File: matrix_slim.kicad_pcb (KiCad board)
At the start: 2 copper layers, 84 x 62.3 mm, 66 parts, among them J2 C168688, SW1 PG1316M, SW10 PG1316S, SW11 PG1316S, SW12 PG1316S, SW13 PG1316S, SW14 PG1316S, SW15 PG1316M, SW16 PG1316M, SW17 PG1316S, SW18 PG1316M, SW2 PG1316M, SW3 PG1316M, SW4 PG1316M, SW5 PG1316M, SW6 PG1316S, SW7 PG1316S, SW8 PG1316S, SW9 PG1316S, U1 nRF52840, U2 BQ24075RGT, U3 XC6220B331MR, Y1 FC-12M, Y2 23MHz XRCGB32M000F1H50R0

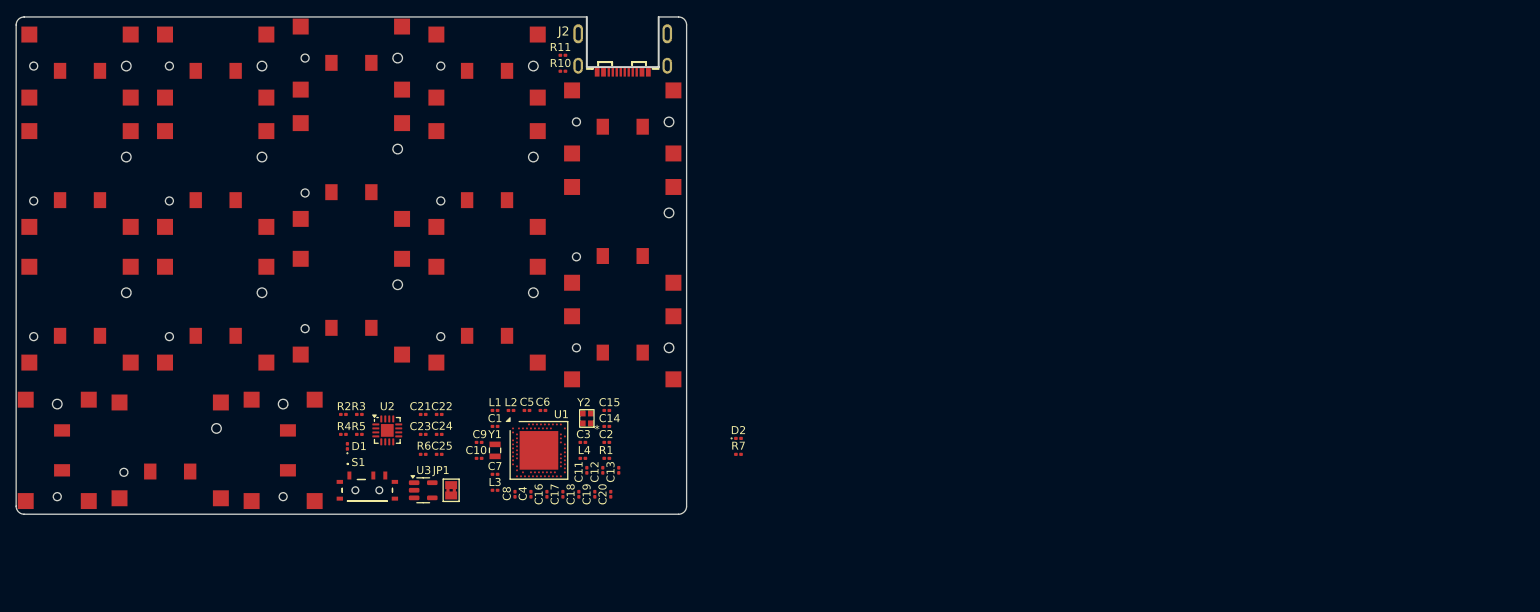
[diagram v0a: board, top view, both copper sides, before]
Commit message: Added base setup
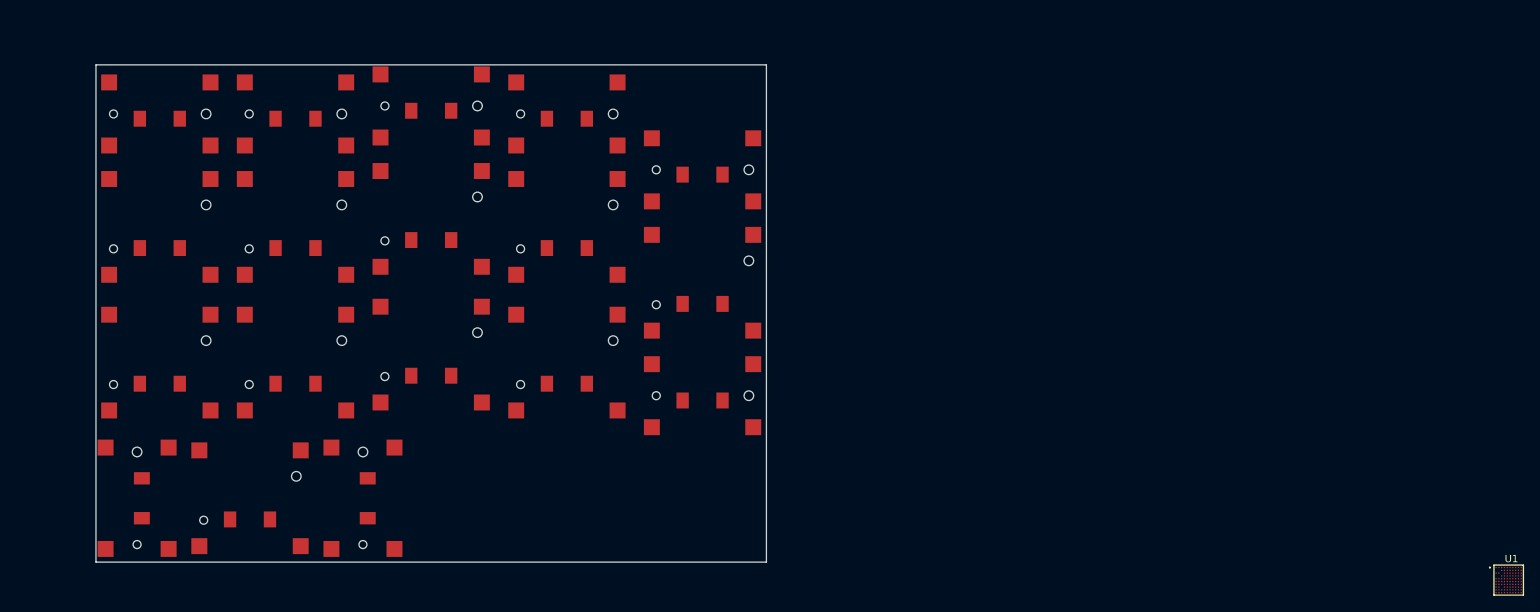
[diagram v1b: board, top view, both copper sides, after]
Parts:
- removed C1, C17, C18, C19: 100nF, Capacitor_SMD:C_0201_0603Metric
- removed C10, C14, C15, C9: 12pF, Capacitor_SMD:C_0201_0603Metric
- removed C11, C12: 1pF, Capacitor_SMD:C_0201_0603Metric
- removed C13: 1.5pF, Capacitor_SMD:C_0201_0603Metric
- removed C16, C21, C6: 1uF, Capacitor_SMD:C_0201_0603Metric
- removed C2: 100pF, Capacitor_SMD:C_0201_0603Metric
- removed C20, C22, C23, C4, C7, C8: 4.7uF, Capacitor_SMD:C_0201_0603Metric
- removed C24: 10uF, Capacitor_SMD:C_0201_0603Metric
- removed C25: 4.7nF, Capacitor_SMD:C_0201_0603Metric
- removed C3: 820pF, Capacitor_SMD:C_0201_0603Metric
- removed C5: 47nF, Capacitor_SMD:C_0201_0603Metric
- removed D1: RED, LED_SMD:LED_0201_0603Metric
- removed D2: BLUE, LED_SMD:LED_0201_0603Metric
- removed J2: C168688, custom_footprints:C168688
- removed JP1: Charge Boost, Jumper:SolderJumper-2_P1.3mm_Bridged2Bar_Pad1.0x1.5mm
- removed L1, L3: 10uH, Inductor_SMD:L_0201_0603Metric
- removed L2: 15nH, Inductor_SMD:L_0201_0603Metric
- removed L4: 3.9nH, Inductor_SMD:L_0201_0603Metric
- removed R1: 0, Resistor_SMD:R_0201_0603Metric
- removed R10, R11: 5.1k, Resistor_SMD:R_0201_0603Metric
- removed R2, R4, R5: 10k, Resistor_SMD:R_0201_0603Metric
- removed R3: 2k, Resistor_SMD:R_0201_0603Metric
- removed R6: 10M, Resistor_SMD:R_0201_0603Metric
- removed R7: 1k, Resistor_SMD:R_0201_0603Metric
- removed S1: MSK12C02, custom_footprints:MSK12C02
- removed U2: BQ24075RGT, Package_DFN_QFN:VQFN-16-1EP_3x3mm_P0.5mm_EP1.6x1.6mm
- removed U3: XC6220B331MR, Package_TO_SOT_SMD:SOT-23-5
- removed Y1: FC-12M, Crystal:Crystal_SMD_3215-2Pin_3.2x1.5mm
- removed Y2: 23MHz XRCGB32M000F1H50R0, custom_footprints:XRCGB32M000F1H01R0
- SW1, SW15, SW16, SW18, SW3, SW4, SW5: footprint custom_footprints:CPG1316M01D02 -> PG1316M:PG1316M
- SW10, SW11, SW12, SW13, SW14, SW17, SW7, SW8, SW9: footprint custom_footprints:CPG1316S01D02 -> PG1316S:PG1316S
- SW2: value PG1316M -> PG1316S; footprint custom_footprints:CPG1316M01D02 -> PG1316S:PG1316S
- SW6: value PG1316S -> PG1316M; footprint custom_footprints:CPG1316S01D02 -> PG1316M:PG1316M
- U1: value nRF52840 -> NRF52840-CKAA-R; footprint Package_DFN_QFN:Nordic_AQFN-73-1EP_7x7mm_P0.5mm -> NRF52840-CKAA-R:NRF52840-CKAA-R
- moved U1 122.6 mm to (207.0, 95.3)
- moved SW6 78.0 mm to (106.0, 43.9)
- moved SW2 21.3 mm to (38.0, 51.0)
- moved SW1 11.7 mm to (38.0, 36.9)
- moved SW10 11.7 mm to (106.0, 58.0)
- moved SW11 11.7 mm to (38.0, 68.0)
- moved SW12 11.7 mm to (55.0, 68.0)
- moved SW13 11.7 mm to (72.0, 67.0)
- moved SW14 11.7 mm to (89.0, 68.0)
- moved SW15 11.7 mm to (106.0, 72.2)
- moved SW16 11.7 mm to (35.1, 85.0)
- moved SW17 11.7 mm to (49.3, 85.0)
- moved SW18 11.7 mm to (63.5, 85.0)
- moved SW7 11.7 mm to (55.0, 51.0)
- moved SW8 11.7 mm to (72.0, 50.0)
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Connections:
- SW1 pad 2: SGND -> GND
- SW1 pad 3: FGND -> SGND
- SW10 pad 2: SGND -> GND
- SW10 pad 3: FGND -> SGND
- SW11 pad 2: SGND -> GND
- SW11 pad 3: FGND -> SGND
- SW12 pad 2: SGND -> GND
- SW12 pad 3: FGND -> SGND
- SW13 pad 2: SGND -> GND
- SW13 pad 3: FGND -> SGND
- SW14 pad 2: SGND -> GND
- SW14 pad 3: FGND -> SGND
- SW15 pad 2: SGND -> GND
- SW15 pad 3: FGND -> SGND
- SW16 pad 2: SGND -> GND
- SW16 pad 3: FGND -> SGND
- SW17 pad 2: SGND -> GND
- SW17 pad 3: FGND -> SGND
- SW18 pad 2: SGND -> GND
- SW18 pad 3: FGND -> SGND
- SW2 pad 2: SGND -> GND
- SW2 pad 3: FGND -> SGND
- SW3 pad 2: SGND -> GND
- SW3 pad 3: FGND -> SGND
- SW4 pad 2: SGND -> GND
- SW4 pad 3: FGND -> SGND
- SW5 pad 2: SGND -> GND
- SW5 pad 3: FGND -> SGND
- SW6 pad 2: SGND -> GND
- SW6 pad 3: FGND -> SGND
- SW7 pad 2: SGND -> GND
- SW7 pad 3: FGND -> SGND
- SW8 pad 2: SGND -> GND
- SW8 pad 3: FGND -> SGND
- SW9 pad 2: SGND -> GND
- SW9 pad 3: FGND -> SGND
- U1 pad A10: 029 -> unconnected-(U1-DEC1-PadA10)
- U1 pad A8: 031 -> unconnected-(U1-DEC4-PadA8)
- U1 pad B3: Net-(U1-DCC) -> unconnected-(U1-VDD-PadB3)
- U1 pad B5: Net-(U1-DEC4) -> unconnected-(U1-P1.14-PadB5)
- U1 pad B7: SGND -> unconnected-(U1-VSS-PadB7)
- U1 pad C1: Net-(U1-DEC1) -> unconnected-(U1-VSS_PA-PadC1)
- U1 pad F2: Net-(U1-XL2/P0.01) -> unconnected-(U1-DEC5/NC-PadF2)
- U1 pad G1: 026 -> unconnected-(U1-P1.07-PadG1)
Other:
- outline, holes or cut-outs redrawn
